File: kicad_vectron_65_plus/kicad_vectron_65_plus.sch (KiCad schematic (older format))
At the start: 31 parts

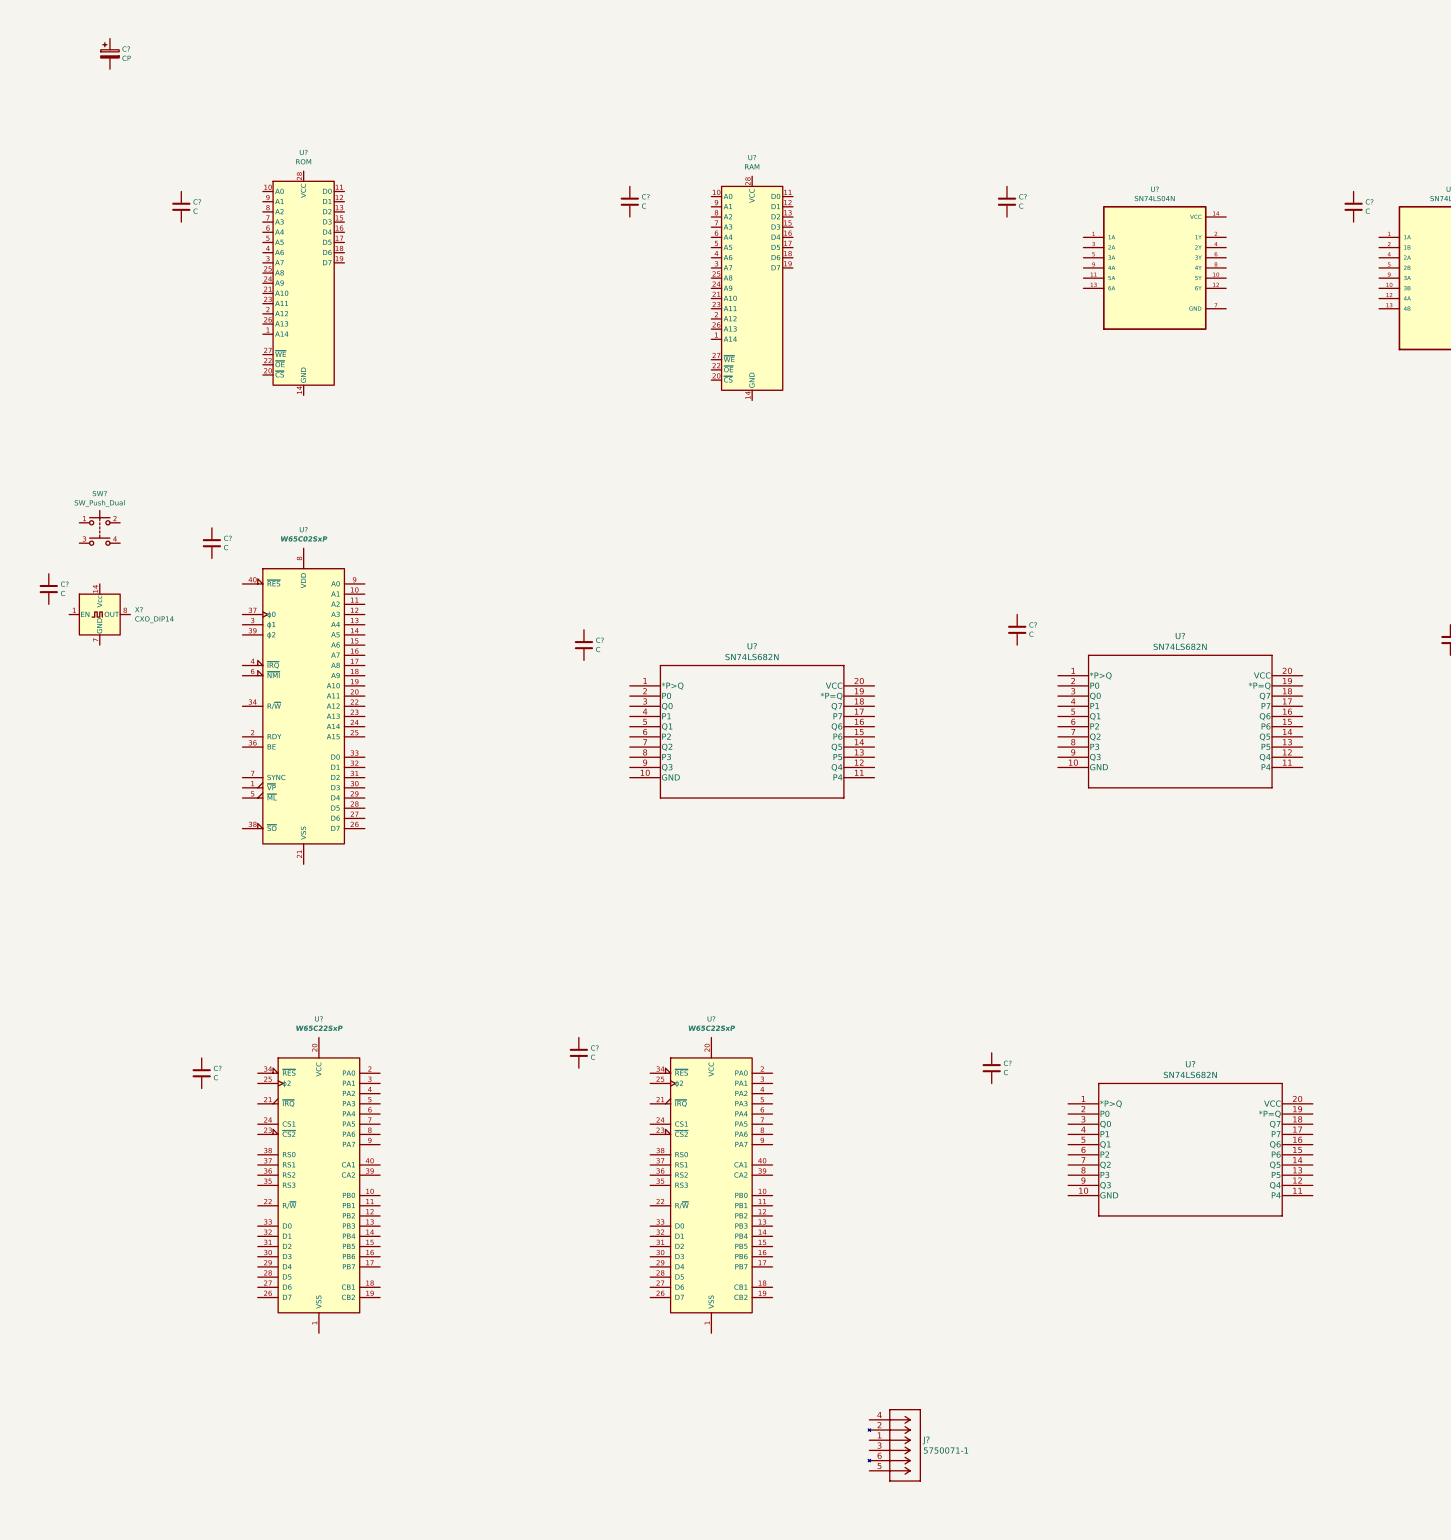
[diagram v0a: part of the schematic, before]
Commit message: Update schematic.
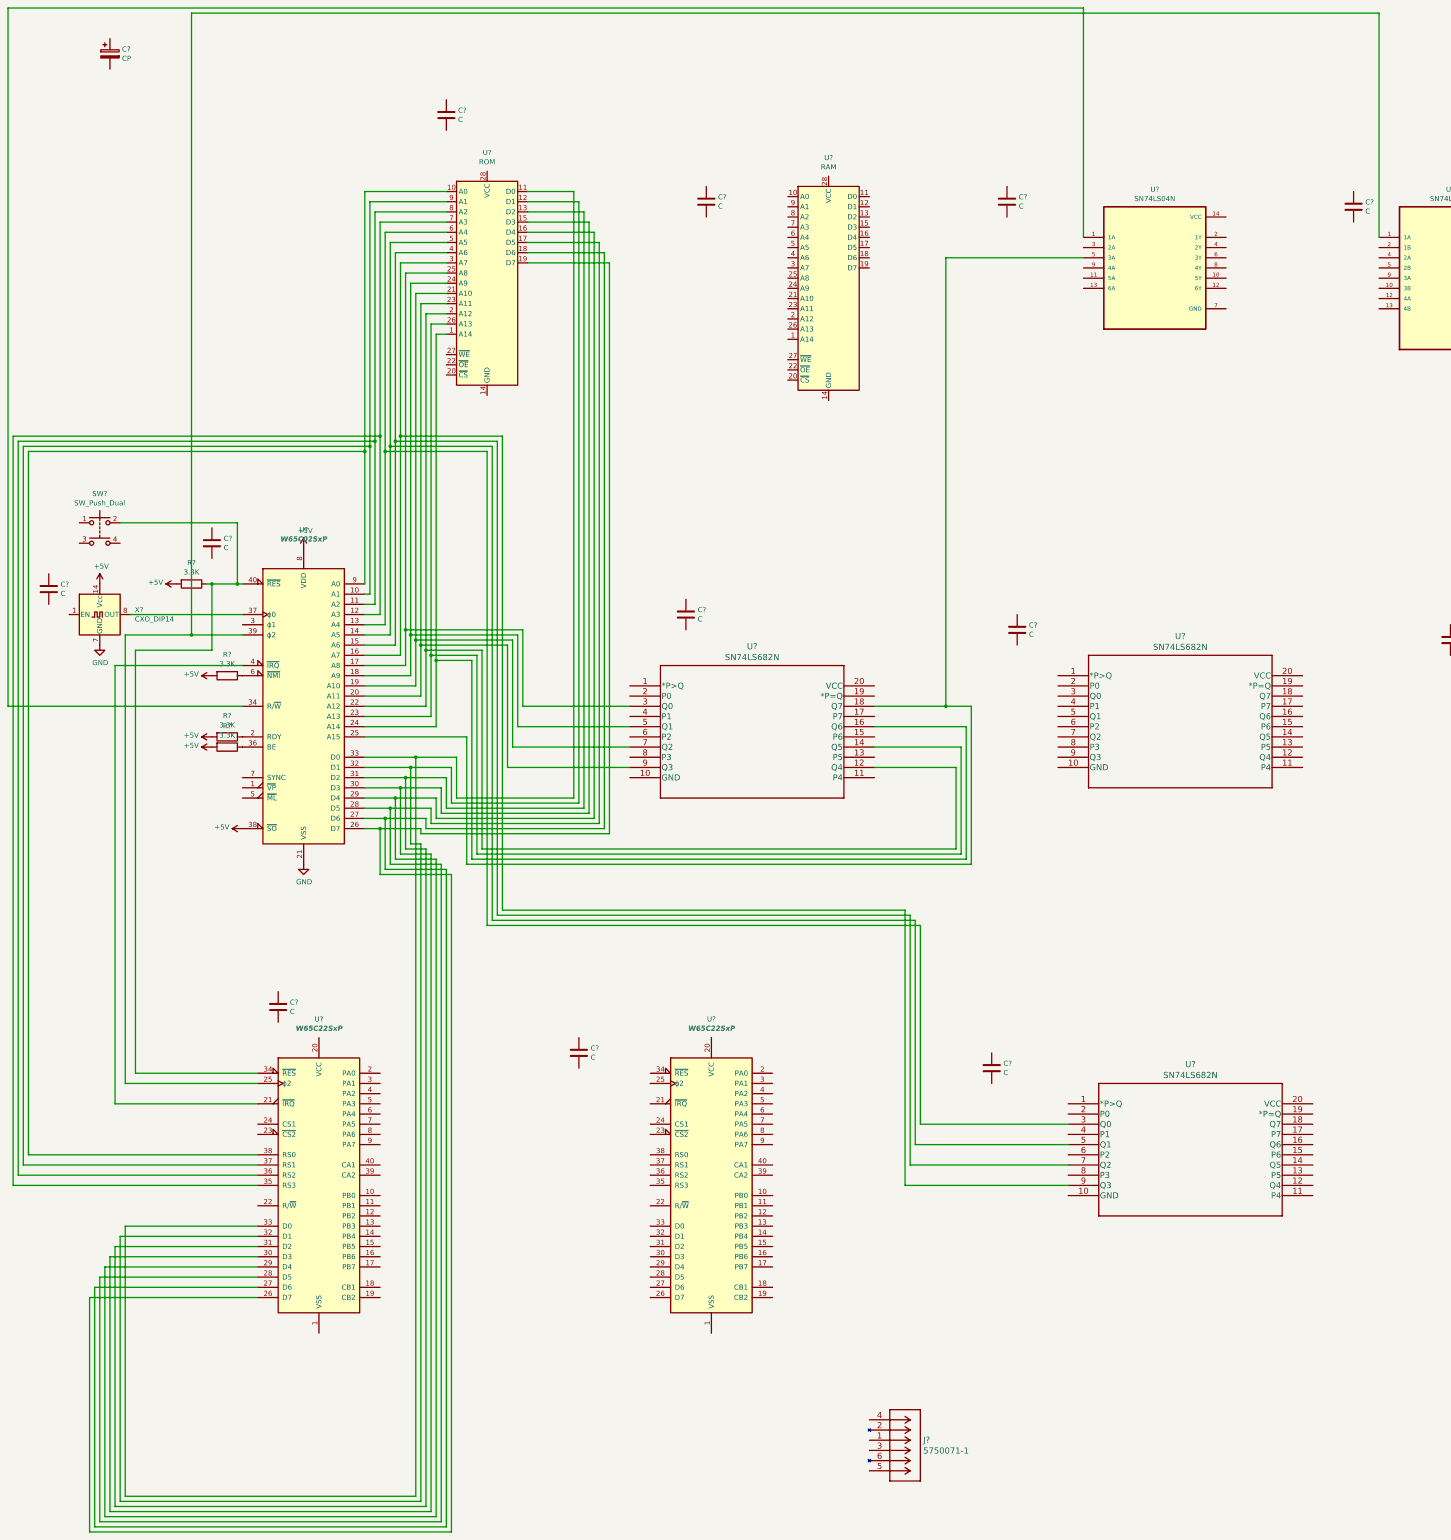
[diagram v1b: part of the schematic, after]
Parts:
- added R? (x4): 3.3K, symbol Device:R
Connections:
- net at U?.10 (A1): now also U?.37 (RS1), U?.9 (A1)
- net at U?.11 (A2): now also U?.36 (RS2), U?.8 (A2)
- net at U?.12 (A3): now also U?.35 (RS3), U?.7 (A3)
- net at U?.13 (A4): now also U?.3 (Q0), U?.6 (A4)
- net at U?.14 (A5): now also U?.5 (A5), U?.5 (Q1)
- net at U?.15 (A6): now also U?.4 (A6), U?.7 (Q2)
- net at U?.16 (A7): now also U?.3 (A7), U?.9 (Q3)
- net at U?.17 (A8): now also U?.25 (A8), U?.3 (Q0)
- net at U?.18 (A9): now also U?.24 (A9), U?.5 (Q1)
- net at U?.19 (A10): now also U?.21 (A10), U?.7 (Q2)
- net at U?.2 (RDY): now also R?.1
- net at U?.20 (A11): now also U?.23 (A11), U?.9 (Q3)
- net GND: now reaches U?.21 (VSS)
- net GND: now also X?.7 (GND)
- net at U?.22 (A12): now also U?.12 (Q4), U?.2 (A12)
- net at U?.23 (A13): now also U?.14 (Q5), U?.26 (A13)
- net at U?.24 (A14): now also U?.1 (A14), U?.16 (Q6)
- net at U?.25 (A15): now also U?.18 (Q7), U?.5 (3A)
- net at U?.26 (D7): now also U?.19 (D7), U?.26 (D7)
- net at U?.27 (D6): now also U?.18 (D6), U?.27 (D6)
- net at U?.28 (D5): now also U?.17 (D5), U?.28 (D5)
- net at U?.29 (D4): now also U?.16 (D4), U?.29 (D4)
- net at U?.30 (D3): now also U?.15 (D3), U?.30 (D3)
- net at U?.31 (D2): now also U?.13 (D2), U?.31 (D2)
- net at U?.32 (D1): now also U?.12 (D1), U?.32 (D1)
- net at U?.33 (D0): now also U?.11 (D0), U?.33 (D0)
- net at U?.34 (R/~W): now also U?.1 (1A)
- net at U?.36 (BE): now also R?.1
- net at U?.37 (ϕ0): now also X?.8 (OUT)
- net +5V: now reaches U?.38 (~SO)
- net +5V: now also U?.8 (VDD), X?.14 (Vcc), R?.2, R?.2, R?.2, R?.2
- net at U?.39 (ϕ2): now also U?.1 (1A), U?.25 (ϕ2)
- net at U?.4 (~IRQ): now also U?.21 (~IRQ)
- net at U?.40 (~RES): now also SW?.2, U?.34 (~RES), R?.1
- net at U?.6 (~NMI): now also R?.1
- net at U?.9 (A0): now also U?.10 (A0), U?.38 (RS0)
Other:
- moved on the sheet: C?, U?

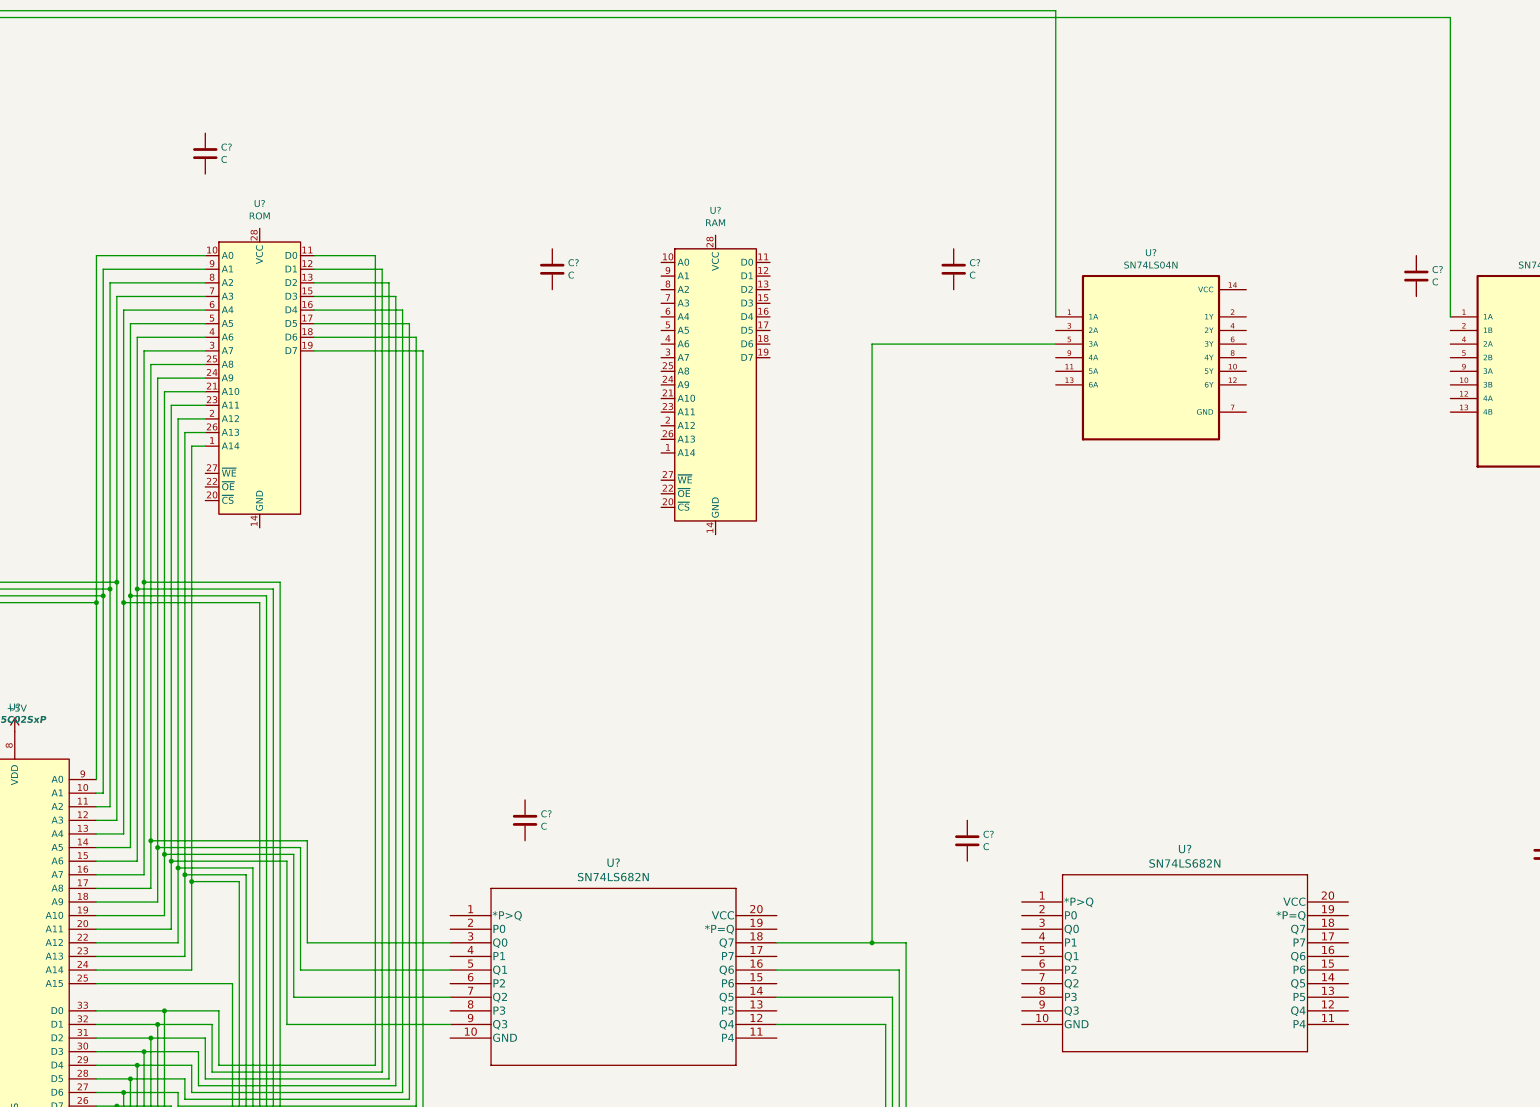
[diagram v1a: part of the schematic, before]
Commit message: Save progress on schematic.
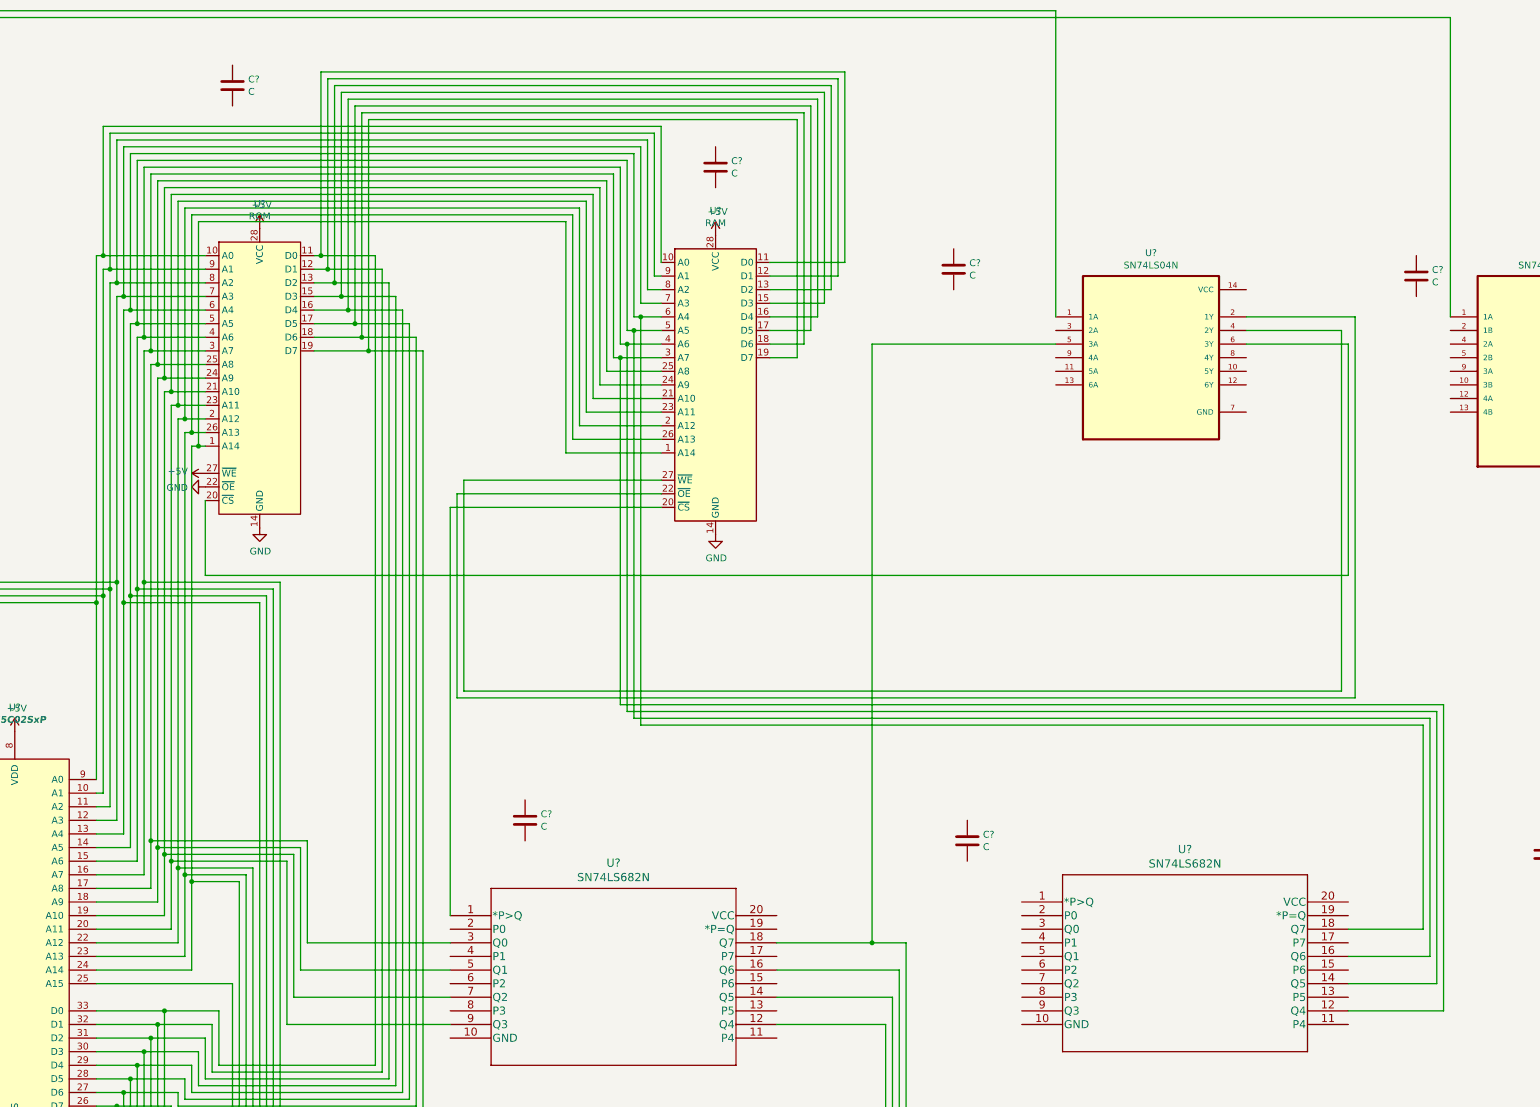
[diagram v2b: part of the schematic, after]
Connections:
- net +5V: now also U?.27 (~WE), U?.28 (VCC), U?.28 (VCC)
- net GND: now also U?.14 (GND), U?.14 (GND), U?.22 (~OE)
- net at U?.10 (A1), U?.37 (RS1), U?.9 (A1): now also U?.9 (A1)
- net at U?.11 (A2), U?.36 (RS2), U?.8 (A2): now also U?.8 (A2)
- net at U?.12 (A3), U?.35 (RS3), U?.7 (A3): now also U?.7 (A3)
- net at U?.13 (A4), U?.3 (Q0), U?.6 (A4): now also U?.18 (Q7), U?.6 (A4)
- net at U?.14 (A5), U?.5 (A5), U?.5 (Q1): now also U?.16 (Q6), U?.5 (A5)
- net at U?.15 (A6), U?.4 (A6), U?.7 (Q2): now also U?.14 (Q5), U?.4 (A6)
- net at U?.16 (A7), U?.3 (A7), U?.9 (Q3): now also U?.12 (Q4), U?.3 (A7)
- net at U?.17 (A8), U?.25 (A8), U?.3 (Q0): now also U?.25 (A8)
- net at U?.18 (A9), U?.24 (A9), U?.5 (Q1): now also U?.24 (A9)
- net at U?.19 (A10), U?.21 (A10), U?.7 (Q2): now also U?.21 (A10)
- net at U?.20 (A11), U?.23 (A11), U?.9 (Q3): now also U?.23 (A11)
- net at U?.12 (Q4), U?.2 (A12), U?.22 (A12): now also U?.2 (A12)
- net at U?.14 (Q5), U?.23 (A13), U?.26 (A13): now also U?.26 (A13)
- net at U?.1 (A14), U?.16 (Q6), U?.24 (A14): now also U?.1 (A14)
- net at U?.19 (D7), U?.26 (D7), U?.26 (D7): now also U?.19 (D7)
- net at U?.18 (D6), U?.27 (D6), U?.27 (D6): now also U?.18 (D6)
- net at U?.17 (D5), U?.28 (D5), U?.28 (D5): now also U?.17 (D5)
- net at U?.16 (D4), U?.29 (D4), U?.29 (D4): now also U?.16 (D4)
- net at U?.15 (D3), U?.30 (D3), U?.30 (D3): now also U?.15 (D3)
- net at U?.13 (D2), U?.31 (D2), U?.31 (D2): now also U?.13 (D2)
- net at U?.12 (D1), U?.32 (D1), U?.32 (D1): now also U?.12 (D1)
- net at U?.11 (D0), U?.33 (D0), U?.33 (D0): now also U?.11 (D0)
- net at U?.10 (A0), U?.38 (RS0), U?.9 (A0): now also U?.10 (A0)
- net at U?.20 (~CS): now also U?.6 (3Y)
- net at U?.20 (~CS): now also U?.1 (*P>Q)
- net at U?.22 (~OE): now also U?.2 (1Y)
- net at U?.27 (~WE): now also U?.4 (2Y)
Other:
- moved on the sheet: C?
